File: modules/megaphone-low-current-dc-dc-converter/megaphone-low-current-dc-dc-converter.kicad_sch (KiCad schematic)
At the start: 9 parts, among them U1 TPS631000DRLR

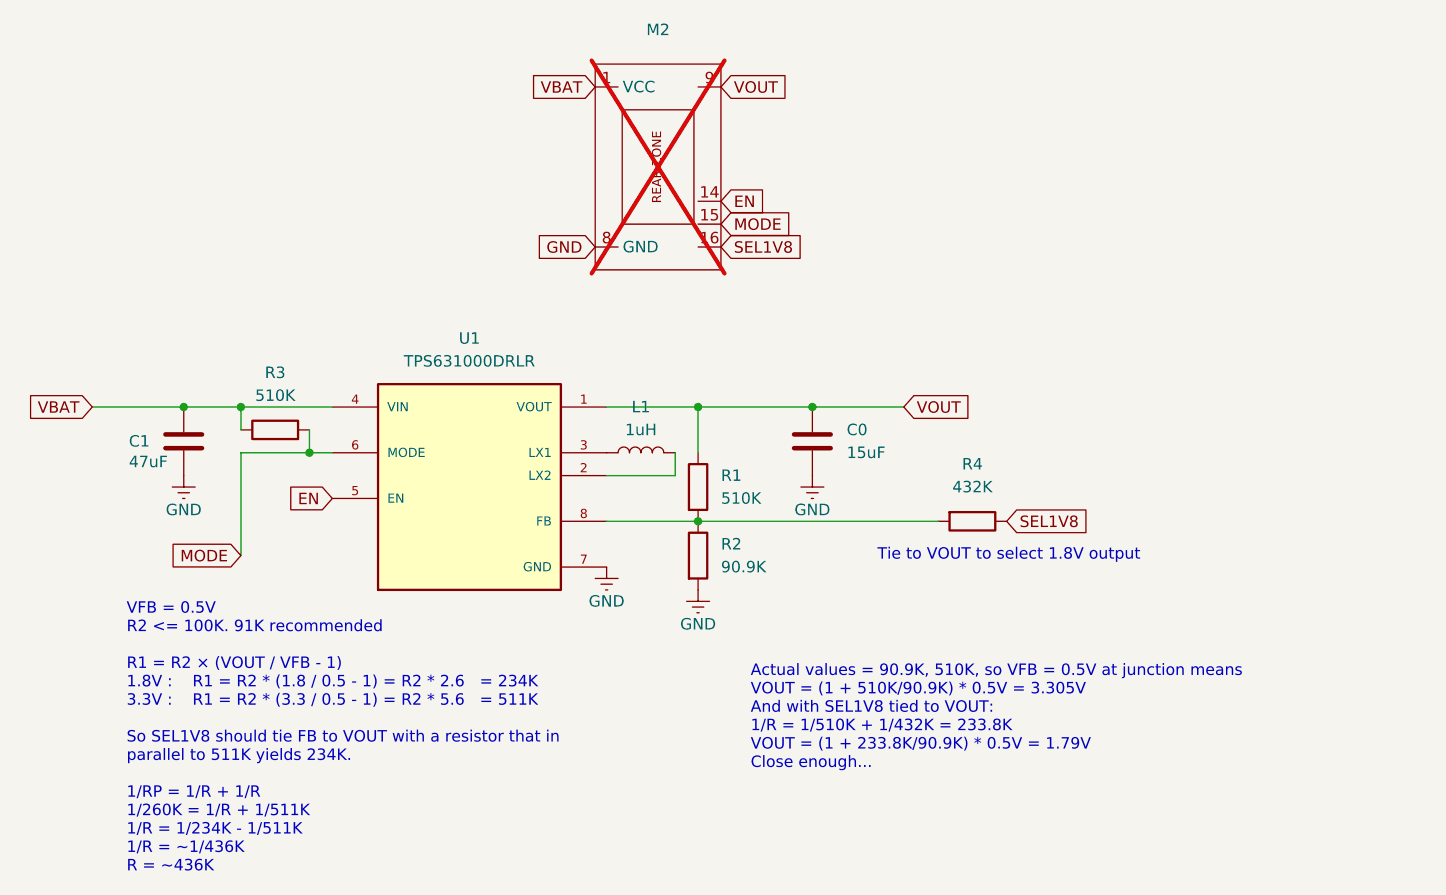
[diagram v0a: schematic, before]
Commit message: Updating all modules
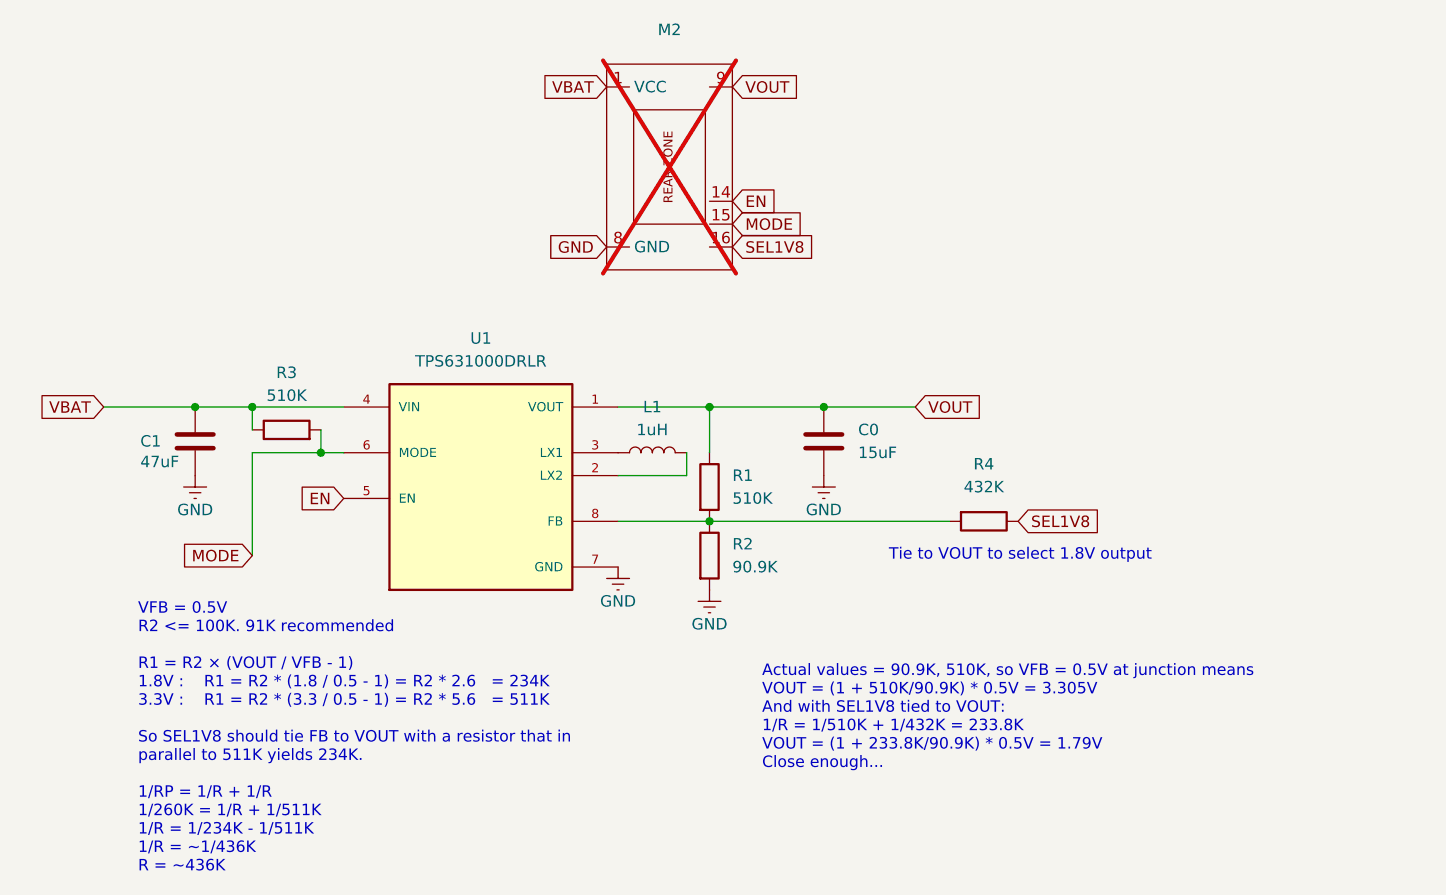
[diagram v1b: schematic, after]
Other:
- moved on the sheet: C0, C1, L1, M2, R1, R2, R3, R4, U1
